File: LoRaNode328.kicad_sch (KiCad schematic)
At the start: 0 parts

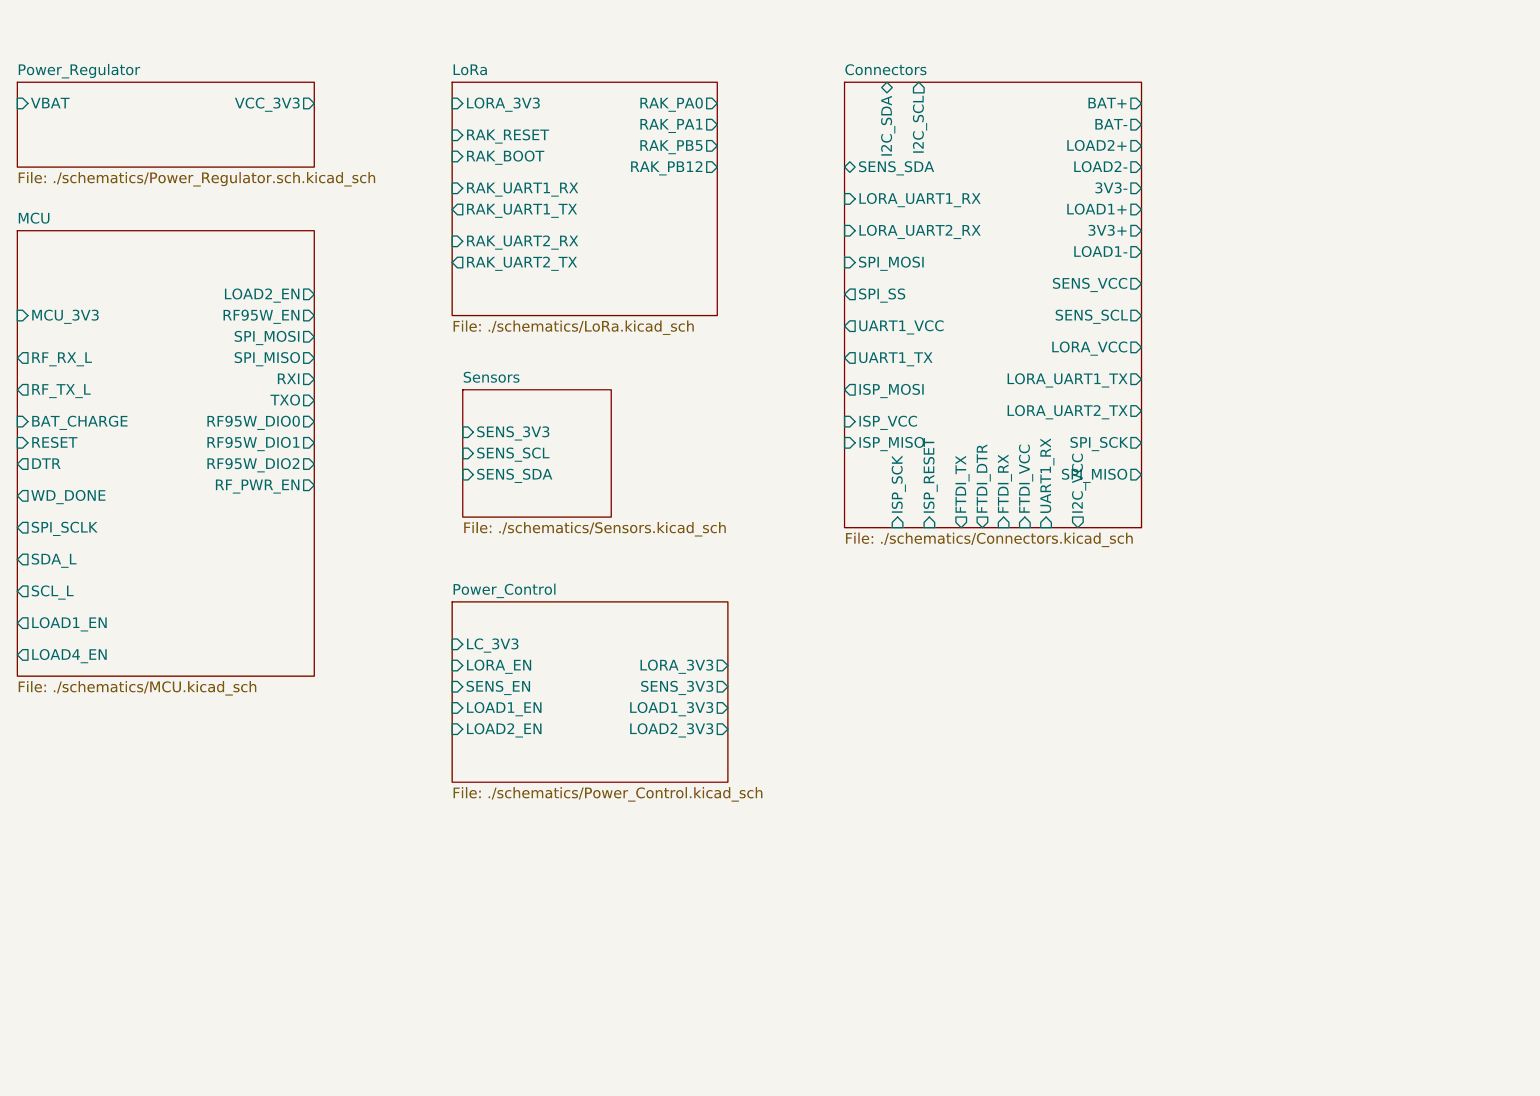
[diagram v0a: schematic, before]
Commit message: root scheme
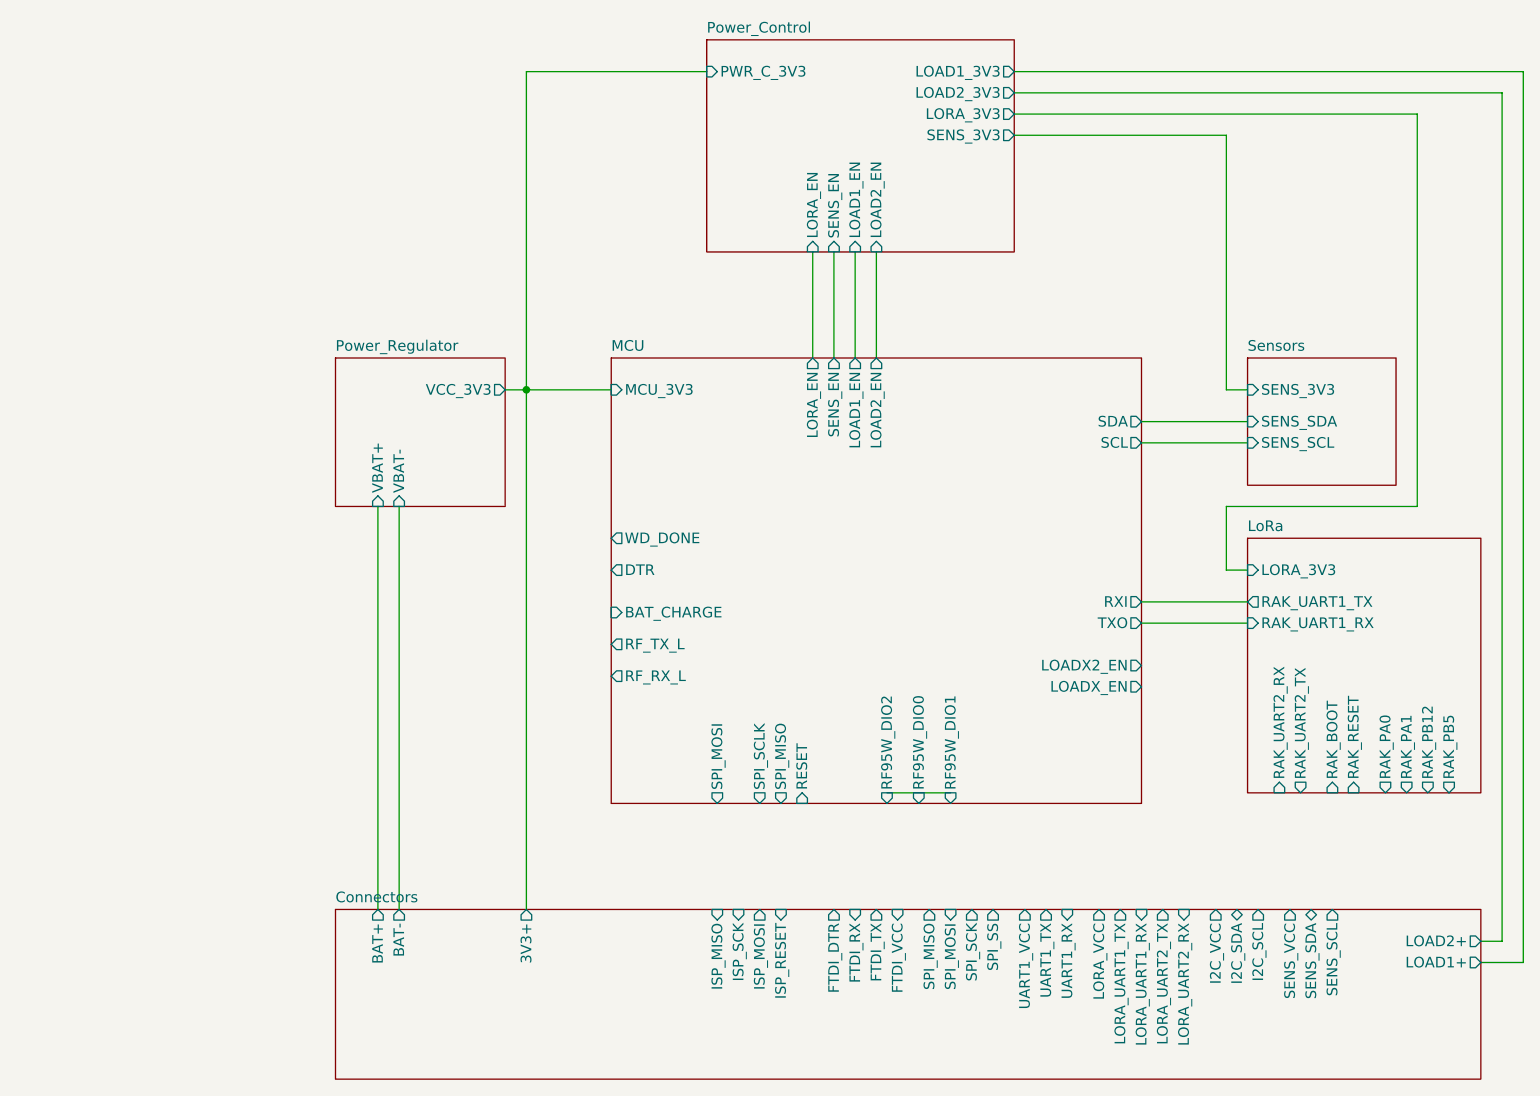
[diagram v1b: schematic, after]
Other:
- sheet Connectors ports: added none; removed 3V3-, ISP_VCC, LOAD1-, LOAD2-
- sheet MCU ports: added LOADX2_EN, LOADX_EN, LORA_EN, SCL, SDA, SENS_EN; removed LOAD4_EN, RF95W_EN, RF_PWR_EN, SCL_L, SDA_L
- sheet Power_Control ports: added PWR_C_3V3; removed LC_3V3
- sheet Power_Regulator ports: added VBAT+, VBAT-; removed VBAT
